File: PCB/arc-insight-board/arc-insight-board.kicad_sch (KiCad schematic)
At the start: 40 parts, among them J1 USB_C_Receptacle, J2 Conn_01x06, J3 Conn_01x05, J4 Conn_01x02, J5 Conn_01x02, J6 FPC_24PIN, J7 Conn_01x02, J8 U.FL, M1 Electret, U1 ESP32-S3, U2 MAX98357A, U3 MAX98357A, U4 TP4054, U5 Comparator, U6 ME6211C33M5, Y1 40MHz

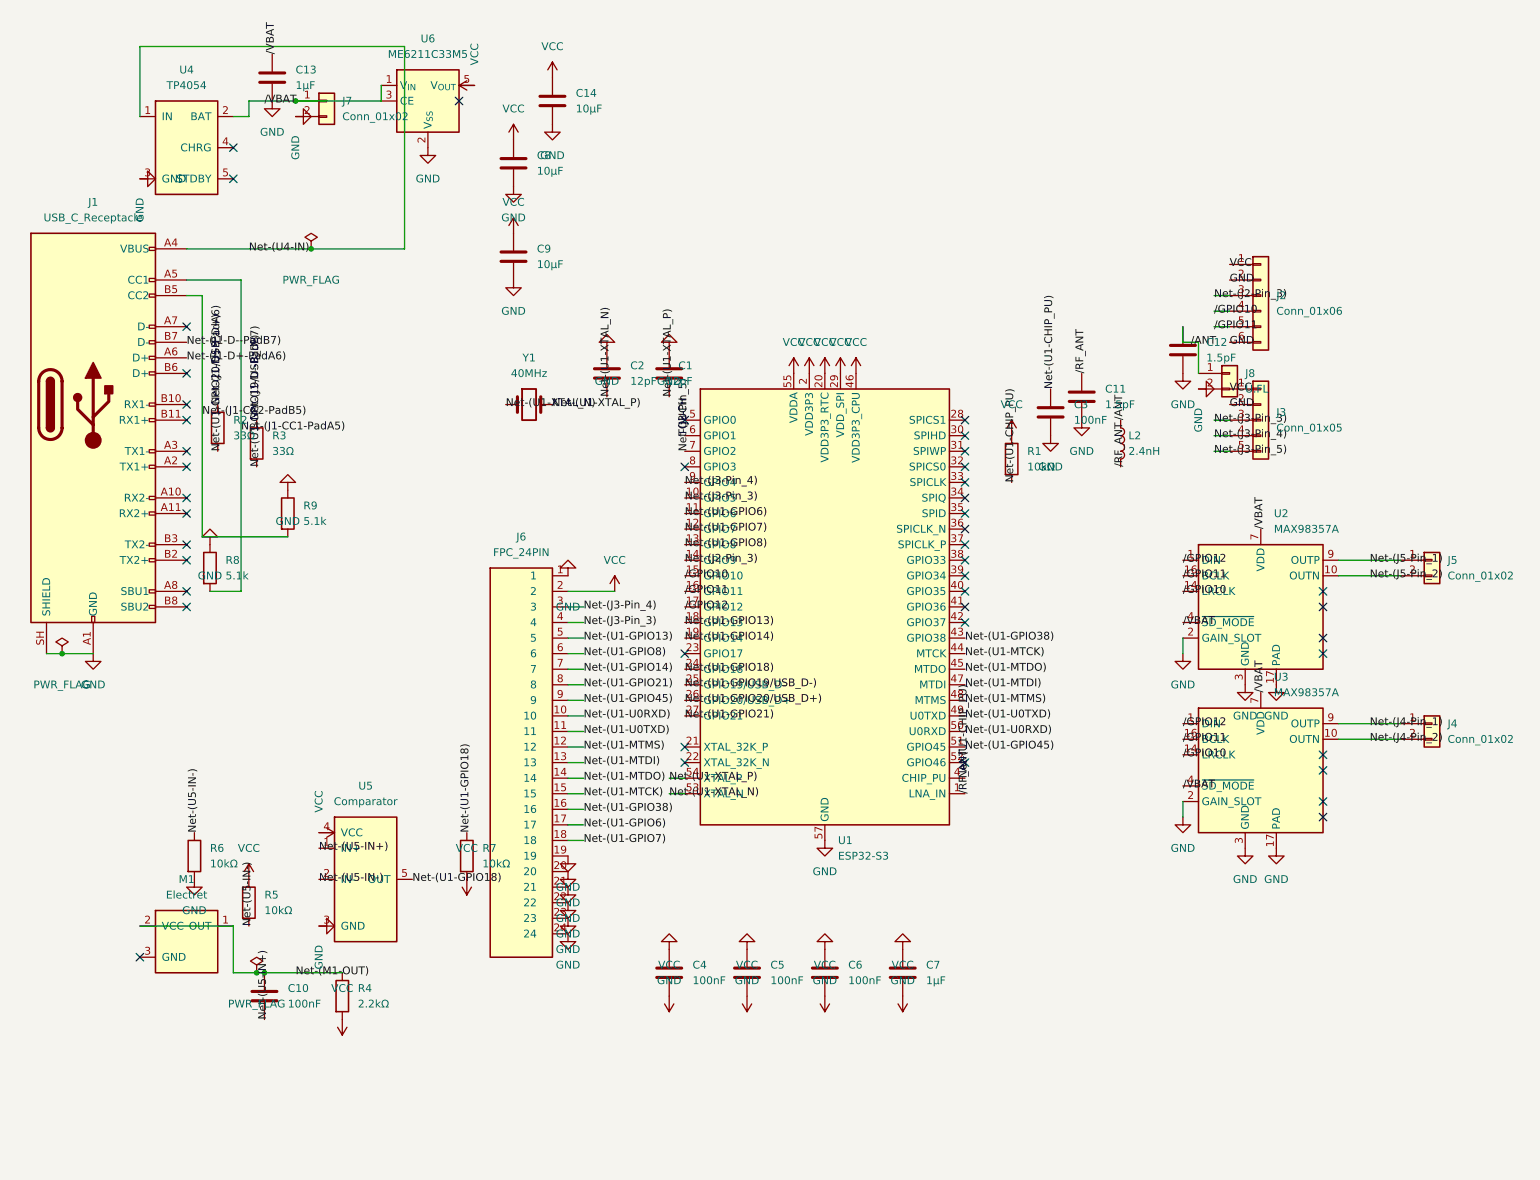
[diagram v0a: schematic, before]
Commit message: Edited files
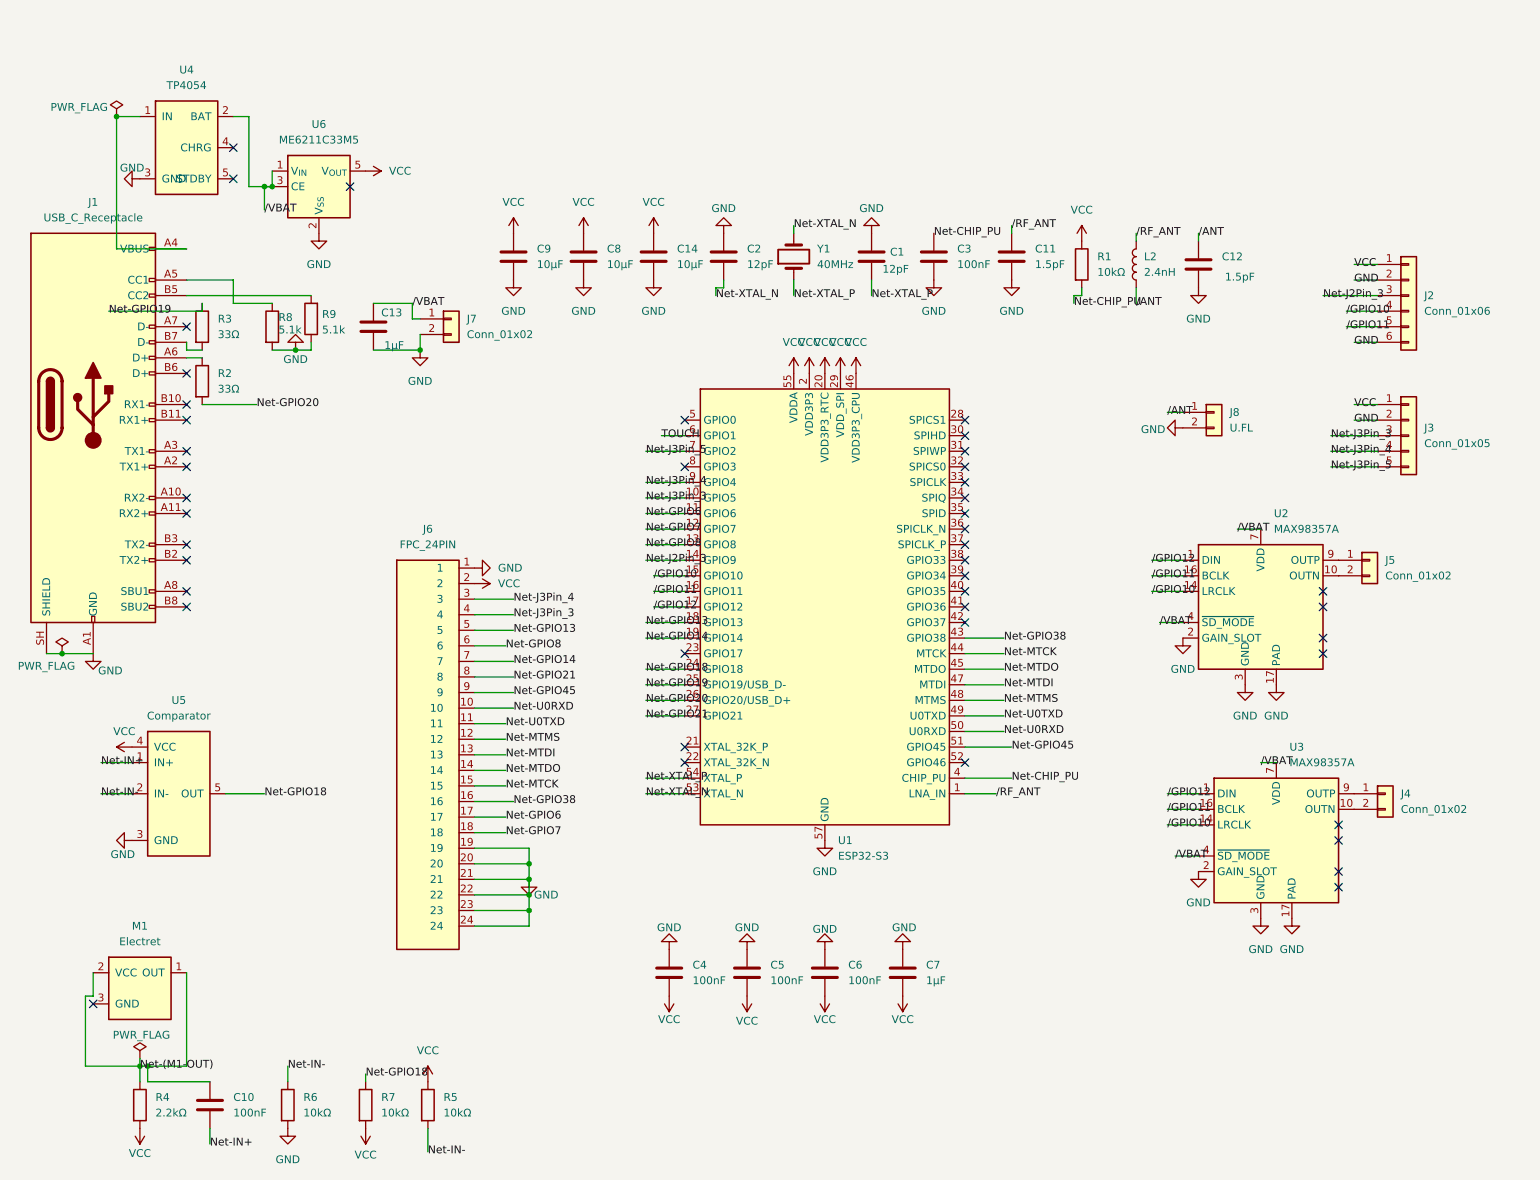
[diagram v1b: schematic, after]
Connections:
- net GND: now also R8.2; no longer R8.1
- net Net-(J1-CC1-PadA5): no longer names the net of J1.A5 (CC1)
- net Net-(J1-CC1-PadA5): now also R8.1; no longer R8.2
- net Net-(J1-CC2-PadB5): no longer names the net of J1.B5 (CC2), R9.2
- net Net-(J1-D+-PadA6): no longer names the net of J1.A6 (D+), R2.1
- net Net-(J1-D--PadB7): no longer names the net of J1.B7 (D-)
- net Net-(J1-D--PadB7): now also R3.2; no longer R3.1
- net Net-(J2-Pin_3) renamed Net-J2Pin_3
- net Net-(J3-Pin_3) renamed Net-J3Pin_3
- net Net-(J3-Pin_4) renamed Net-J3Pin_4
- net Net-(J3-Pin_5) renamed Net-J3Pin_5
- net Net-(J4-Pin_1): no longer names the net of J4.1 (Pin_1), U3.9 (OUTP)
- net Net-(J4-Pin_2): no longer names the net of J4.2 (Pin_2), U3.10 (OUTN)
- net Net-(J5-Pin_1): no longer names the net of J5.1 (Pin_1), U2.9 (OUTP)
- net Net-(J5-Pin_2): no longer names the net of J5.2 (Pin_2), U2.10 (OUTN)
- net Net-(U1-CHIP_PU) renamed Net-CHIP_PU
- net Net-(U1-GPIO13) renamed Net-GPIO13
- net Net-(U1-GPIO14) renamed Net-GPIO14
- net Net-(U1-GPIO18) renamed Net-GPIO18
- net Net-(U1-GPIO19/USB_D-) renamed Net-GPIO19
- net Net-GPIO19: now also R3.1; no longer R3.2
- net Net-(U1-GPIO20/USB_D+) renamed Net-GPIO20
- net Net-(U1-GPIO21) renamed Net-GPIO21
- net Net-(U1-GPIO38) renamed Net-GPIO38
- net Net-(U1-GPIO45) renamed Net-GPIO45
- net Net-(U1-GPIO6) renamed Net-GPIO6
- net Net-(U1-GPIO7) renamed Net-GPIO7
- net Net-(U1-GPIO8) renamed Net-GPIO8
- net Net-(U1-MTCK) renamed Net-MTCK
- net Net-(U1-MTDI) renamed Net-MTDI
- net Net-(U1-MTDO) renamed Net-MTDO
- net Net-(U1-MTMS) renamed Net-MTMS
- net Net-(U1-U0RXD) renamed Net-U0RXD
- net Net-(U1-U0TXD) renamed Net-U0TXD
- net Net-(U1-XTAL_N) renamed Net-XTAL_N
- net Net-XTAL_N: now also Y1.2; no longer Y1.1
- net Net-(U1-XTAL_P) renamed Net-XTAL_P
- net Net-XTAL_P: now also Y1.1; no longer Y1.2
- net Net-(U4-IN): no longer names the net of J1.A4 (VBUS), J1.A9 (VBUS), J1.B4 (VBUS), J1.B9 (VBUS), U4.1 (IN)
- net Net-(U5-IN+) renamed Net-IN+
- net Net-(U5-IN-) renamed Net-IN-
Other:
- moved on the sheet: C1, C10, C11, C12, C13, C14, C2, C3, C8, J2, J3, J4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
